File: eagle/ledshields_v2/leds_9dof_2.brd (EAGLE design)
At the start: 20 x 42 mm, 14 parts, among them J1 J5MM, U3 PCA9685

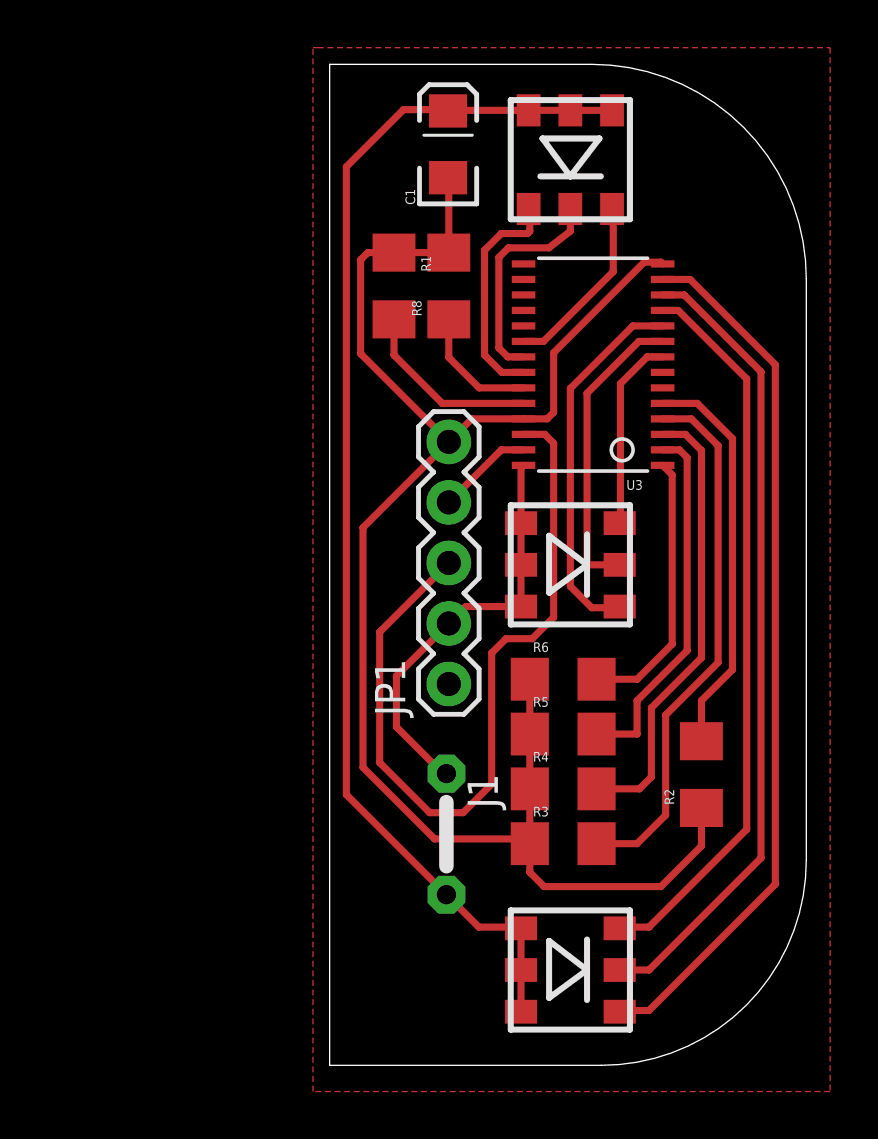
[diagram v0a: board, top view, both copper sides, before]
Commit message: modified 2nd version pcb designs for milling
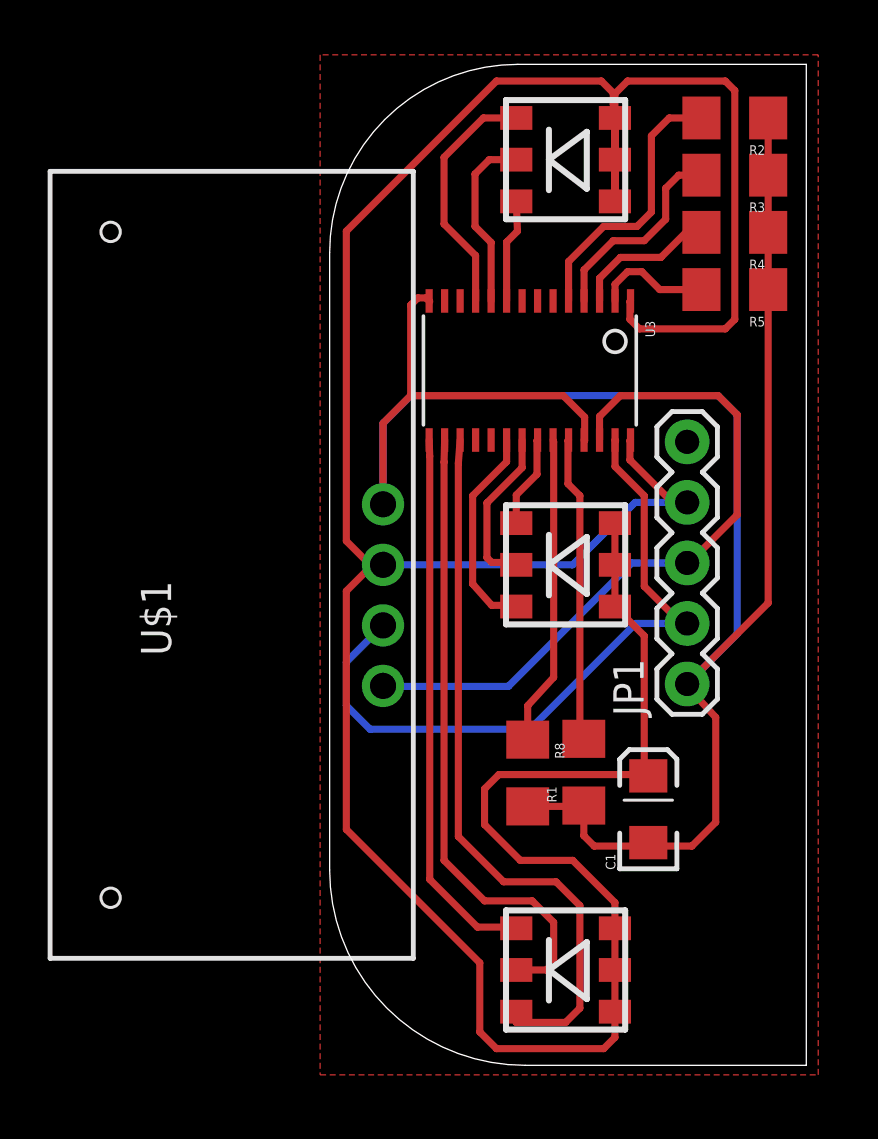
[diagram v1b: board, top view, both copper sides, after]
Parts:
- removed J1: J5MM, jumper:05
- removed R6: 10K, SparkFun-Resistors:1206
- added U$1: LSM9DS0_BREAKOUT, Mlab_ProEx2015:LSM9DS0_BREAKOUT
- moved C1 29.1 mm to (13.4, 10.7)
- moved R3 29.0 mm to (17.0, 37.4), turned to 180 degrees
- moved R2 27.6 mm to (17.0, 39.8), turned to 180 degrees
- moved R4 24.4 mm to (17.0, 35.0), turned to 180 degrees
- moved R1 21.9 mm to (10.7, 12.3), turned to 90 degrees
- moved R8 20.7 mm to (8.31, 12.3), turned to 270 degrees
- moved R5 20.0 mm to (17.0, 32.5), turned to 180 degrees
- moved LED1 17.0 mm to (9.90, 21.0), turned to 90 degrees
- moved LED2 17.0 mm to (9.90, 38.0), turned to 90 degrees
- moved JP1 10.0 mm to (15.0, 16.0)
- moved U3 2.67 mm to (8.40, 29.2), turned to 180 degrees
- moved LED3 0.20 mm to (9.90, 4.00), turned to 90 degrees
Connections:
- removed net A0: R6.2, U3.1
- removed net GPIO: JP1.1
- new net INT: JP1.5
- net 3.3V: now also JP1.4, U$1.VDD, U3.1; no longer J1.1, J1.2, JP1.2
- net GND: now also JP1.1, U$1.GND; no longer JP1.5, R6.1
- net PWM10: now also LED3.BC
- net PWM2: no longer LED2.BC
- net PWM3: now also LED2.BC; no longer LED2.RC
- net PWM4: now also LED2.RC; no longer LED2.GC
- net PWM5: now also LED2.GC; no longer LED3.BC
- net PWM6: no longer LED3.RC
- net PWM7: no longer LED3.GC
- net PWM8: now also LED3.GC
- net PWM9: now also LED3.RC
- net SCL: now also U$1.SCL
- net SDA: now also JP1.2, U$1.SDA; no longer JP1.4
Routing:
- net 3.3V: track 69.3 -> 137.8 mm
- net PWM7: track 36.8 -> 0.00 mm
- net PWM6: track 33.7 -> 0.00 mm
- net PWM10: track 0.00 -> 30.6 mm
- net PWM9: track 0.00 -> 26.7 mm
- net SDA: track 4.05 -> 29.7 mm
- net PWM8: track 0.00 -> 22.9 mm
- net PWM5: track 30.7 -> 10.3 mm
- net GND: track 71.1 -> 91.0 mm
- net A3: track 22.6 -> 8.64 mm
- net A2: track 19.0 -> 6.02 mm
- net A0: track 11.5 -> 0.00 mm
- net A1: track 15.5 -> 4.86 mm
- net PWM3: track 12.6 -> 4.37 mm
- net PWM4: track 15.7 -> 7.59 mm
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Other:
- outline, holes or cut-outs redrawn
